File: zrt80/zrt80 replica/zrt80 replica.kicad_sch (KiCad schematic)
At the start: 108 parts, among them J1 VIDEO, J2 POWER, J3 KEYBOARD, J4 S2-S3, J5 RS232, J6 CHAR, J7 RAM, Q1 2N2222, Q2 2N5484, Y1 20MHz, Y2 2.4576MHz

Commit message: schematic 'done'
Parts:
- removed J5: RS232, symbol Connector_Generic:Conn_02x13_Odd_Even
- added J5: RS232, Connector_PinHeader_2.54mm:PinHeader_2x13_P2.54mm_Vertical, symbol Connector_Generic:Conn_02x13_Top_Bottom
- C1, C10, C11, C12, C13, C14, C15, C16, C17, C18, C19, C2, C20, C21, C22, C24, C25, C26, C27, C28, C29, C30, C31, C32, C33, C34, C35, C36, C4, C5, C6, C9: footprint (none) -> Evan's parts:C_Disc_D6.0mm_W2.5mm_P6.35mm
- C23: footprint (none) -> Evan's parts:trimmer cap
- C3: footprint (none) -> Capacitor_THT:CP_Radial_D10.0mm_P5.00mm
- C7, C8: footprint (none) -> Capacitor_THT:C_Disc_D4.3mm_W1.9mm_P5.00mm
- D1: footprint (none) -> LED_THT:LED_D5.0mm
- D2: footprint Diode_THT:D_DO-35_SOD27_P7.62mm_Horizontal -> Diode_THT:D_DO-35_SOD27_P12.70mm_Horizontal
- J1: footprint (none) -> Connector_PinHeader_2.54mm:PinHeader_2x05_P2.54mm_Vertical
- J2: footprint (none) -> TerminalBlock_Phoenix:TerminalBlock_Phoenix_MKDS-1,5-8-5.08_1x08_P5.08mm_Horizontal
- J3: footprint (none) -> Connector_PinHeader_2.54mm:PinHeader_2x13_P2.54mm_Vertical
- J4: footprint (none) -> Connector_PinHeader_2.54mm:PinHeader_2x10_P2.54mm_Vertical
- J6: footprint (none) -> Connector_PinHeader_2.54mm:PinHeader_1x03_P2.54mm_Vertical
- J7: footprint (none) -> Connector_PinHeader_2.54mm:PinHeader_1x06_P2.54mm_Vertical
- L1: footprint (none) -> Inductor_THT:L_Axial_L9.5mm_D4.0mm_P15.24mm_Horizontal_Fastron_SMCC
- Q1: footprint Package_TO_SOT_THT:TO-92_Inline -> Package_TO_SOT_THT:TO-5-3
- Q2: footprint TRANS_2N5484 -> Package_TO_SOT_THT:TO-92L_Inline_Wide
- R1, R10, R11, R12, R13, R14, R15, R16, R17, R2, R3, R4, R5, R6, R7, R8, R9: footprint (none) -> Evan's parts:R_Axial_DIN0204_L3.6mm_D1.6mm_P12.7mm_Horizontal
- S1, S2, S3: footprint (none) -> Button_Switch_THT:SW_DIP_SPSTx08_Slide_6.7x21.88mm_W7.62mm_P2.54mm_LowProfile
- TP1: footprint (none) -> TestPoint:TestPoint_Plated_Hole_D2.0mm
- Y1: footprint (none) -> Crystal:Crystal_HC49-U_Vertical
- Y2: footprint (none) -> Crystal:Crystal_HC33-U_Vertical
- Z1, Z16, Z17, Z2, Z28, Z4: footprint (none) -> Package_DIP:DIP-14_W7.62mm
- Z10, Z11, Z18, Z20, Z21, Z22, Z23, Z29, Z37: footprint (none) -> Package_DIP:DIP-16_W7.62mm
- Z12: footprint (none) -> Package_DIP:DIP-40_W15.24mm
- Z14: footprint DIP254P762X469-14 -> Package_DIP:DIP-14_W7.62mm
- Z15: footprint DIP794W45P254L1969H508Q14 -> Package_DIP:DIP-14_W7.62mm
- Z26, Z27: footprint (none) -> Package_DIP:DIP-18_W7.62mm
- Z31, Z36, Z6, Z7, Z9: footprint (none) -> Package_DIP:DIP-20_W7.62mm
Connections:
- net at R16.1: now also C36.2, Z28.9
- net GND: now reaches R16.2
- net GND: now also C1.2, C10.2, C11.2, C12.2, C13.2, C14.2, C15.2, C16.2, C17.2, C18.2, C19.2, C2.2, C21.2, C22.2, C23.2, C24.2, C25.2, C26.2, C27.2, C28.2, C29.2, C3.2, C30.2, C31.2, C32.2, C33.2, C34.2, C35.2, C4.2, C5.2, C6.2, C7.2, C8.2, C9.2, J1.1 (Pin_1), J1.3 (Pin_3), J1.5 (Pin_5), J1.7 (Pin_7), J1.9 (Pin_9), J2.2 (Pin_2), J2.5 (Pin_5), J3.10 (Pin_10), J3.12 (Pin_12), J3.14 (Pin_14), J3.16 (Pin_16), J3.2 (Pin_2), J3.21 (Pin_21), J3.4 (Pin_4), J3.6 (Pin_6), J3.8 (Pin_8), J4.1 (Pin_1), J4.2 (Pin_2), J7.3 (Pin_3), J7.6 (Pin_6), Q2.1, R12.1, R17.2, R6.1, S1.1, S1.2, S1.3, S1.4, S1.5, S1.6, S1.7, S2.1, S2.2, S2.3, S2.4, S2.5, S2.6, S2.7, S2.8, S3.1, S3.2, S3.3, S3.4, S3.5, S3.6, S3.7, S3.8, Z1.7 (GND), Z10.14 (Cext), Z10.6 (Cext), Z10.8 (GND), Z11.8 (GND), Z12.29 (GND), Z13.19 (WR), Z13.20 (GND), Z13.22 (RD), Z13.25 (~{ADS}), Z14.7 (GND), Z15.7 (GND), Z16.7 (GND), Z17.7 (GND), Z18.8 (GND), Z19.1 (GND), Z19.3 (LPSTB), Z2.7 (GND), Z20.15 (E), Z20.8 (GND), Z21.15 (E), Z21.8 (GND), Z22.15 (E), Z22.8 (GND), Z23.15 (E), Z23.8 (GND), Z24.12 (GND), Z25.12 (GND), Z26.9 (Gnd), Z27.9 (Gnd), Z28.7 (GND), Z29.1 (Ds), Z29.6 (CE), Z29.8 (GND), Z30.12 (GND), Z30.18 (~{CE}), Z30.20 (~{OE}/VPP), Z31.1 (OE), Z31.10 (GND), Z32.12 (GND), Z32.20 (~{OE}), Z33.12 (GND), Z33.20 (~{OE}), Z34.12 (GND), Z34.20 (~{OE}), Z35.12 (GND), Z35.20 (~{OE}), Z36.10 (GND), Z37.15 (E), Z37.8 (GND), Z4.7 (GND), Z6.10 (GND), Z7.10 (GND), J5.7 (Pin_7)
- net at C20.1: now also C22.1, R12.2, R13.1, Z13.16 (XIN)
- net at C20.2: now also Y2.1
- net at Y2.2: now also R13.2, Z13.17 (XOUT), Z28.1
- net I/O4: now reaches Z9.1 (OEa)
- net I/O4: now also Z11.11 (O4), Z9.19 (OEb)
- net D3: now reaches Z9.12 (O3a)
- net D3: now also Z12.8 (D3), Z13.4 (D3), Z19.30 (D3), Z24.13 (D3), Z25.13 (D3), Z26.14 (D0), Z36.14 (B4), Z6.12 (O3a), Z7.12 (O3a)
- net D2: now reaches Z9.14 (O2a)
- net D2: now also Z12.12 (D2), Z13.3 (D2), Z19.31 (D2), Z24.11 (D2), Z25.11 (D2), Z26.13 (D1), Z36.11 (B7), Z6.14 (O2a), Z7.14 (O2a)
- net D1: now reaches Z9.16 (O1a)
- net D1: now also Z12.15 (D1), Z13.2 (D1), Z19.32 (D1), Z24.10 (D1), Z25.10 (D1), Z26.12 (D2), Z36.12 (B6), Z6.16 (O1a), Z7.16 (O1a)
- net D0: now reaches Z9.18 (O0a)
- net D0: now also Z12.14 (D0), Z13.1 (D0), Z19.33 (D0), Z24.9 (D0), Z25.9 (D0), Z26.11 (D3), Z36.13 (B5), Z6.18 (O0a), Z7.18 (O0a)
- net +5V: now reaches Z9.20 (VCC)
- net +5V: now also C1.1, C10.1, C11.1, C12.1, C13.1, C14.1, C15.1, C16.1, C17.1, C18.1, C19.1, C2.1, C21.1, C24.1, C25.1, C26.1, C27.1, C28.1, C29.1, C30.1, C31.1, C32.1, C33.1, C34.1, C35.1, C4.1, C5.1, C6.1, C9.1, D2.1 (K), J2.3 (Pin_3), J3.24 (Pin_24), J3.25 (Pin_25), J3.26 (Pin_26), J6.1 (Pin_1), L1.1, Q1.3 (C), R1.2, R10.2, R11.2, R14.2, R15.2, R2.2, R7.2, R8.2, R9.2, Z1.14 (VCC), Z10.10 (B), Z10.11 (Clr), Z10.16 (VCC), Z10.2 (B), Z10.3 (Clr), Z11.16 (VCC), Z12.11 (VCC), Z13.12 (CS0), Z13.13 (CS1), Z13.40 (VCC), Z14.14 (VCC), Z16.14 (VCC), Z17.14 (VCC), Z18.16 (VCC), Z19.20 (VCC), Z19.23 (E), Z2.14 (VCC), Z20.16 (VCC), Z21.16 (VCC), Z22.16 (VCC), Z23.16 (VCC), Z24.24 (VCC), Z25.24 (VCC), Z26.18 (Vcc), Z27.18 (Vcc), Z28.14 (VCC), Z29.16 (VCC), Z3.1 (R1.1), Z30.24 (VCC), Z31.20 (VCC), Z32.24 (VCC), Z33.24 (VCC), Z34.24 (VCC), Z35.24 (VCC), Z36.20 (VCC), Z37.16 (VCC), Z4.14 (VCC), Z5.1 (R1.1), Z6.20 (VCC), Z7.20 (VCC), Z8.1 (R1.1)
- net D7: now reaches Z9.3 (O3b)
- net D7: now also Z12.13 (D7), Z13.8 (D7), Z19.26 (D7), Z24.17 (D7), Z25.17 (D7), Z27.14 (D0), Z36.18 (B0), Z6.3 (O3b), Z7.3 (O3b)
- net D6: now reaches Z9.5 (O2b)
- net D6: now also Z12.10 (D6), Z13.7 (D6), Z19.27 (D6), Z24.16 (D6), Z25.16 (D6), Z27.13 (D1), Z36.17 (B1), Z6.5 (O2b), Z7.5 (O2b)
- net D5: now reaches Z9.7 (O1b)
- net D5: now also Z12.9 (D5), Z13.6 (D5), Z19.28 (D5), Z24.15 (D5), Z25.15 (D5), Z27.12 (D2), Z36.16 (B2), Z6.7 (O1b), Z7.7 (O1b)
- net D4: now reaches Z9.9 (O0b)
- net D4: now also Z12.7 (D4), Z13.5 (D4), Z19.29 (D4), Z24.14 (D4), Z25.14 (D4), Z27.11 (D3), Z36.15 (B3), Z6.9 (O0b), Z7.9 (O0b)
- net cSyncPol: now reaches Z3.2 (R1.2)
- net cSyncPol: now also S1.16, Z2.1
- net -12V: now reaches Z15.1 (VCC-)
- net -12V: now also J2.1 (Pin_1), J3.22 (Pin_22), J3.23 (Pin_23)
- net at Z15.10 (3B): now also Z13.32 (~{RTS}), Z15.9 (3A)
- net TxDATA: now reaches Z15.11 (4Y)
- net TxDATA: now also J5.2 (Pin_2)
- net at Z15.12 (4A): now also Z13.11 (SOUT), Z15.13 (4B)
- net +12V: now reaches Z15.14 (VCC_+)
- net +12V: now also J2.4 (Pin_4), J3.19 (Pin_19), J3.20 (Pin_20)
- net at Z15.4 (2A): now also Z13.33 (~{DTR}), Z15.5 (2B)
- net DTR: now reaches Z15.6 (2Y)
- net DTR: now also J5.20 (Pin_20)
- net RTS: now reaches Z15.8 (3Y)
- net RTS: now also J5.4 (Pin_4)
- net bell: now reaches Z10.12 (~{Q})
- net bell: now also Z16.2
- net at Z10.7 (RCext): now also C7.1, R8.1
- net I/O6: now reaches Z10.9 (A)
- net I/O6: now also Z11.9 (O6)
- net RAM A7: now reaches Z33.1 (A7)
- net RAM A7: now also Z22.12 (Zd), Z32.1 (A7), Z34.1 (A7), Z35.1 (A7)
- net RAM D1: now reaches Z33.10 (Q1)
- net RAM D1: now also Z31.4 (D1), Z32.10 (Q1), Z34.10 (Q1), Z35.10 (Q1), Z36.8 (A6)
- net RAM D2: now reaches Z33.11 (Q2)
- net RAM D2: now also Z31.3 (D0), Z32.11 (Q2), Z34.11 (Q2), Z35.11 (Q2), Z36.9 (A7)
- net RAM D3: now reaches Z33.13 (Q3)
- net RAM D3: now also Z31.8 (D3), Z32.13 (Q3), Z34.13 (Q3), Z35.13 (Q3), Z36.6 (A4)
- net RAM D4: now reaches Z33.14 (Q4)
- net RAM D4: now also Z31.13 (D4), Z32.14 (Q4), Z34.14 (Q4), Z35.14 (Q4), Z36.5 (A3)
- net RAM D5: now reaches Z33.15 (Q5)
- net RAM D5: now also Z31.14 (D5), Z32.15 (Q5), Z34.15 (Q5), Z35.15 (Q5), Z36.4 (A2)
- net RAM D6: now reaches Z33.16 (Q6)
- net RAM D6: now also Z31.17 (D6), Z32.16 (Q6), Z34.16 (Q6), Z35.16 (Q6), Z36.3 (A1)
- net RAM D7: now reaches Z33.17 (Q7)
- net RAM D7: now also Z31.18 (D7), Z32.17 (Q7), Z34.17 (Q7), Z35.17 (Q7), Z36.2 (A0)
- net RAM /CS2: now reaches Z33.18 (~{CS})
- net RAM /CS2: now also Z37.10 (O2)
- net RAM A10: now reaches Z33.19 (A10)
- net RAM A10: now also Z21.9 (Zc), Z32.19 (A10), Z34.19 (A10), Z35.19 (A10)
- net RAM A6: now reaches Z33.2 (A6)
- net RAM A6: now also Z22.9 (Zc), Z32.2 (A6), Z34.2 (A6), Z35.2 (A6)
- net RAM /WR: now reaches Z33.21 (~{WE})
- net RAM /WR: now also Z21.12 (Zd), Z32.21 (~{WE}), Z34.21 (~{WE}), Z35.21 (~{WE})
- net RAM A9: now reaches Z33.22 (A9)
- net RAM A9: now also Z21.7 (Zb), Z32.22 (A9), Z34.22 (A9), Z35.22 (A9)
- net RAM A8: now reaches Z33.23 (A8)
- net RAM A8: now also Z21.4 (Za), Z32.23 (A8), Z34.23 (A8), Z35.23 (A8)
- net RAM A5: now reaches Z33.3 (A5)
- net RAM A5: now also Z22.7 (Zb), Z32.3 (A5), Z34.3 (A5), Z35.3 (A5)
- net RAM A4: now reaches Z33.4 (A4)
- net RAM A4: now also Z22.4 (Za), Z32.4 (A4), Z34.4 (A4), Z35.4 (A4)
- net RAM A3: now reaches Z33.5 (A3)
- net RAM A3: now also Z23.12 (Zd), Z32.5 (A3), Z34.5 (A3), Z35.5 (A3)
- net RAM A2: now reaches Z33.6 (A2)
- net RAM A2: now also Z23.9 (Zc), Z32.6 (A2), Z34.6 (A2), Z35.6 (A2)
- net RAM A1: now reaches Z33.7 (A1)
- net RAM A1: now also Z23.7 (Zb), Z32.7 (A1), Z34.7 (A1), Z35.7 (A1)
- net RAM A0: now reaches Z33.8 (A0)
- net RAM A0: now also Z23.4 (Za), Z32.8 (A0), Z34.8 (A0), Z35.8 (A0)
- net RAM D0: now reaches Z33.9 (Q0)
- net RAM D0: now also Z31.7 (D2), Z32.9 (Q0), Z34.9 (Q0), Z35.9 (Q0), Z36.7 (A5)
- net SW2-2: now reaches Z5.2 (R1.2)
- net SW2-2: now also J4.14 (Pin_14), S2.15, Z5.3 (R2.2)
- net at R1.1: now also D1.2 (A)
- net at Z13.10 (SIN): now also Z14.6 (OUT_B)
- net I/O0: now reaches Z13.14 (~{CS2})
- net I/O0: now also Z11.15 (O0)
- net at Z13.15 (~{BAUDOUT}): now also Z13.9 (RCLK)
- net /WR: now reaches Z13.18 (~{WR})
- net /WR: now also Z12.22 (~{WR}), Z19.22 (R/~{W}), Z21.14 (I0d), Z26.10 (R/~{W}), Z27.10 (R/~{W}), Z36.1 (A->B)
- net /RD: now reaches Z13.21 (~{RD})
- net /RD: now also Z12.21 (~{RD})
- net A2: now reaches Z13.26 (A2)
- net A2: now also Z12.32 (A2), Z23.11 (I0c), Z24.6 (A2), Z25.6 (A2), Z26.7 (A2), Z27.7 (A2)
- net A1: now reaches Z13.27 (A1)
- net A1: now also Z12.31 (A1), Z23.5 (I0b), Z24.7 (A1), Z25.7 (A1), Z26.6 (A1), Z27.6 (A1)
- net A0: now reaches Z13.28 (A0)
- net A0: now also Z12.30 (A0), Z19.24 (RS), Z23.2 (I0a), Z24.8 (A0), Z25.8 (A0), Z26.5 (A0), Z27.5 (A0)
- net at Z13.30 (INTR): now also Z28.5
- net CA11: now reaches Z13.31 (~{OUT2})
- net CA11: now also J6.3 (Pin_3)
- net at Z13.34 (~{OUT1}): now also Z16.12, Z16.13
- net RESET: now reaches Z13.35 (MR)
- net RESET: now also Z4.11, Z4.12
- net at Z13.36 (~{CTS}): now also Z14.8 (OUT_C)
- net at Z13.37 (~{DSR}): now also Z14.3 (OUT_A)
- net at Z13.38 (~{DCD}): now also Z14.11 (OUT_D)
- net caps lock: now reaches Z13.39 (~{RI})
- net caps lock: now also J3.18 (Pin_18), J4.3 (Pin_3), Z8.10 (R9.2)
- net at Z16.4: now also Z1.12 (Q3), Z1.8 (Cp0)
- net CRTC CLK: now reaches Z16.5
- net CRTC CLK: now also Z1.5 (Q0), Z19.21 (CLK)
- net at Z16.6: now also Z18.9 (Cp), Z4.9
- net SW2-8: now reaches Z5.10 (R9.2)
- net SW2-8: now also J4.8 (Pin_8), S2.9
- net at J6.2 (Pin_2): now also Z30.21 (A11)
- net at Z2.2: now also Z17.3, Z4.5
- net Csync Out: now reaches Z2.3
- net Csync Out: now also J1.8 (Pin_8)
- net at Z3.6 (R5.2): now also Z1.1 (Pl), Z1.13 (Mr)
- net at R4.1: now also Z4.6
- net at R4.2: now also Q1.2 (B), R3.2
- net SW2-4: now reaches J4.10 (Pin_10)
- net SW2-4: now also S2.13, Z5.6 (R5.2)
- net SW3-5: now reaches J4.11 (Pin_11)
- net SW3-5: now also S3.12, Z8.9 (R8.2)
- net SW2-3: now reaches J4.12 (Pin_12)
- net SW2-3: now also S2.14, Z5.5 (R4.2)
- net SW3-1: now reaches J4.13 (Pin_13)
- net SW3-1: now also S3.16, Z8.2 (R1.2)
- net SW3-2: now reaches J4.15 (Pin_15)
- net SW3-2: now also S3.15, Z8.4 (R3.2)
- net SW2-1: now reaches J4.16 (Pin_16)
- net SW2-1: now also S2.16
- net SW3-3: now reaches J4.17 (Pin_17)
- net SW3-3: now also S3.14, Z8.6 (R5.2)
- net SW2-5: now reaches J4.18 (Pin_18)
- net SW2-5: now also S2.12, Z5.7 (R6.2)
- net SW3-4: now reaches J4.19 (Pin_19)
- net SW3-4: now also S3.13, Z8.8 (R7.2)
- net SW2-6: now reaches J4.20 (Pin_20)
- net SW2-6: now also S2.11, Z5.8 (R7.2)
- net EXRESET: now reaches J4.4 (Pin_4)
- net EXRESET: now also C3.1, D2.2 (A), J2.6 (Pin_6), R14.1, S1.11, Z4.13
- net SW3-8: now reaches J4.5 (Pin_5)
- net SW3-8: now also S3.9, Z8.3 (R2.2)
- net SW2-7: now reaches J4.6 (Pin_6)
- net SW2-7: now also S2.10, Z5.9 (R8.2)
- net SW3-7: now reaches J4.7 (Pin_7)
- net SW3-7: now also S3.10, Z8.5 (R4.2)
- net SW3-6: now reaches J4.9 (Pin_9)
- net SW3-6: now also S3.11, Z8.7 (R6.2)
- net hSyncPol: now reaches Z3.7 (R6.2)
- net hSyncPol: now also S1.12, Z2.10
- net KBD0: now reaches J3.1 (Pin_1)
- net KBD0: now also Z7.2 (I0a)
- net KBD5: now reaches J3.11 (Pin_11)
- net KBD5: now also Z7.13 (I1b)
- net KBD6: now reaches J3.13 (Pin_13)
- net KBD6: now also Z7.15 (I2b)
- net ALT: now reaches J3.15 (Pin_15)
- net ALT: now also S1.13, Z3.5 (R4.2), Z7.17 (I3b)
- net KBD STB: now reaches J3.17 (Pin_17)
- net KBD STB: now also Z17.13
- net KBD1: now reaches J3.3 (Pin_3)
- net KBD1: now also Z7.4 (I1a)
- net KBD2: now reaches J3.5 (Pin_5)
- net KBD2: now also Z7.6 (I2a)
- net KBD3: now reaches J3.7 (Pin_7)
- net KBD3: now also Z7.8 (I3a)
- net KBD4: now reaches J3.9 (Pin_9)
- net KBD4: now also Z7.11 (I0b)
- net at Z1.6 (Cp1): now also R2.1, Z28.8
- net Earth_Protective: now reaches TP1.1
- net Earth_Protective: now also J5.1 (Pin_1)
- net A6: now reaches Z27.1 (A6)
- net A6: now also Z12.36 (A6), Z22.11 (I0c), Z24.2 (A6), Z25.2 (A6), Z26.1 (A6)
- net A9: now reaches Z27.15 (A9)
- net A9: now also Z12.39 (A9), Z21.5 (I0b), Z24.22 (A9), Z25.22 (A9), Z26.15 (A9)
- net A8: now reaches Z27.16 (A8)
- net A8: now also Z12.38 (A8), Z21.2 (I0a), Z24.23 (A8), Z25.23 (A8), Z26.16 (A8)
- net A7: now reaches Z27.17 (A7)
- net A7: now also Z12.37 (A7), Z22.14 (I0d), Z24.1 (A7), Z25.1 (A7), Z26.17 (A7)
- net A5: now reaches Z27.2 (A5)
- net A5: now also Z11.3 (A2), Z12.35 (A5), Z22.5 (I0b), Z24.3 (A5), Z25.3 (A5), Z26.2 (A5)
- net A4: now reaches Z27.3 (A4)
- net A4: now also Z11.2 (A1), Z12.34 (A4), Z22.2 (I0a), Z24.4 (A4), Z25.4 (A4), Z26.3 (A4)
- net A3: now reaches Z27.4 (A3)
- net A3: now also Z11.1 (A0), Z12.33 (A3), Z23.14 (I0d), Z24.5 (A3), Z25.5 (A3), Z26.4 (A3)
- net /mem1: now reaches Z27.8 (~{CS})
- net /mem1: now also Z26.8 (~{CS}), Z37.5 (O1)
- net KSTB Pol: now reaches S1.10
- net KSTB Pol: now also Z17.12, Z3.8 (R7.2)
- net vidPol: now reaches S1.14
- net vidPol: now also Z2.12, Z3.4 (R3.2)
- net vSyncPol: now reaches S1.15
- net vSyncPol: now also Z2.4, Z3.3 (R2.2)
- net beep in: now reaches S1.8
- net beep in: now also Z16.3
- net beep out: now reaches S1.9
- net beep out: now also J2.8 (Pin_8)
- net at C23.1: now also C36.1, L1.2, Q2.2, Y1.2
- net /mem0: now reaches Z25.18 (~{CE})
- net /mem0: now also Z24.18 (~{CE}), Z37.4 (O0)
- net A10: now reaches Z25.19 (A10)
- net A10: now also Z12.40 (A10), Z21.11 (I0c), Z24.19 (A10)
- net A12: now reaches Z25.20 (~{OE}/VPP)
- net A12: now also Z12.2 (A12), Z20.5 (I0b), Z28.11
- net A11: now reaches Z25.21 (A11)
- net A11: now also Z12.1 (A11), Z20.2 (I0a), Z24.21 (A11)
- net at Y1.1: now also Q2.3, R17.1
- net I/O3: now reaches Z6.1 (OEa)
- net I/O3: now also Z11.12 (O3), Z6.19 (OEb)
- net phi: now reaches Z28.2
- net phi: now also R15.1, Z12.6 (~{CLK}), Z28.3
- net at R3.1: now also Z4.4
- net CURSOR: now reaches Z17.10
- net CURSOR: now also Z19.19 (CURSOR)
- net at Z17.8: now also Z18.4 (D0)
- net at Z17.9: now also Z31.19 (O7)
- net /phi: now reaches Z28.4
- net DSR: now reaches Z14.1 (IN_A)
- net DSR: now also J5.6 (Pin_6)
- net CTS: now reaches Z14.10 (IN_C)
- net CTS: now also J5.5 (Pin_5)
- net at Z14.12 (RESPONSE_COTROL_D): now also R9.1
- net RLSD: now reaches Z14.13 (IN_D)
- net RLSD: now also J5.8 (Pin_8)
- net at Z14.2 (RESPONSE_COTROL_A): now also R10.1
- net RxDATA: now reaches Z14.4 (IN_B)
- net RxDATA: now also J5.3 (Pin_3)
- net at Z28.10: now also Z24.20 (~{OE}/VPP)
- net at Z4.1: now also Z16.8, Z2.13
- net at Z4.2: now also Z4.3
- net /INT: now reaches Z28.6
- net /INT: now also Z12.16 (~{INT})
- net Vsync: now reaches Z17.1
- net Vsync: now also Z19.40 (VS), Z2.5
- net Hsync: now reaches Z17.2
- net Hsync: now also Z19.39 (HS), Z2.9
- net at Z17.11: now also Z12.17 (~{NMI})
- net Video Out: now reaches Z2.11
- net Video Out: now also J1.2 (Pin_2)
- net /mem3: now reaches Z22.1 (S)
- net /mem3: now also Z18.5 (D1), Z20.1 (S), Z21.1 (S), Z23.1 (S), Z36.19 (CE), Z37.7 (O3)
- net CRTC A6: now reaches Z22.10 (I1c)
- net CRTC A6: now also Z19.10 (MA6)
- net CRTC A7: now reaches Z22.13 (I1d)
- net CRTC A7: now also Z19.11 (MA7)
- net CRTC A4: now reaches Z22.3 (I1a)
- net CRTC A4: now also Z19.8 (MA4)
- net CRTC A5: now reaches Z22.6 (I1b)
- net CRTC A5: now also Z19.9 (MA5)
- net at Z30.1 (A7): now also Z31.9 (O3)
- net at Z30.10 (D1): now also Z29.3 (B)
- net at Z30.11 (D2): now also Z29.4 (C)
- net at Z30.13 (D3): now also Z29.5 (D)
- net at Z30.14 (D4): now also Z29.10 (E)
- net at Z30.15 (D5): now also Z29.11 (F)
- net at Z30.16 (D6): now also Z29.12 (G)
- net at Z30.17 (D7): now also Z29.14 (H)
- net at Z30.19 (A10): now also Z31.16 (O6)
- net at Z30.2 (A6): now also Z31.2 (O0)
- net at Z30.22 (A9): now also Z31.15 (O5)
- net at Z30.23 (A8): now also Z31.12 (O4)
- net at Z30.3 (A5): now also Z31.5 (O1)
- net at Z30.4 (A4): now also Z31.6 (O2)
- net RA3: now reaches Z30.5 (A3)
- net RA3: now also Z19.35 (RA3)
- net RA2: now reaches Z30.6 (A2)
- net RA2: now also Z19.36 (RA2)
- net RA1: now reaches Z30.7 (A1)
- net RA1: now also Z19.37 (RA1)
- net RA0: now reaches Z30.8 (A0)
- net RA0: now also Z19.38 (RA0)
- net at Z30.9 (D0): now also Z29.2 (A)
- net at R11.1: now also Z12.25 (~{BUSRQ})
- net RAM /CS0: now reaches Z35.18 (~{CS})
- net RAM /CS0: now also Z37.12 (O0)
- net at Z17.4: now also Z18.2 (Q0)
- net raw video: now reaches Z17.5
- net raw video: now also Z29.13 (Qh)
- net at Z17.6: now also Z16.9
- net Vsync Out: now reaches Z2.6
- net Vsync Out: now also J1.6 (Pin_6)
- net I/O7: now reaches Z10.1 (A)
- net I/O7: now also Z11.7 (O7)
- net at Z10.15 (RCext): now also C8.1, R7.1
- net beep: now reaches Z10.4 (~{Q})
- net beep: now also Z16.1
- net /RESET: now reaches Z4.10
- net /RESET: now also Z12.26 (~{RESET})
- net at R5.1: now also Q1.1 (E), R6.2
- net composite video: now reaches R5.2
- net composite video: now also J1.10 (Pin_10)
- net at Z5.4 (R3.2): now also Z21.13 (I1d)
- net CRTC A13: now reaches Z20.10 (I1c)
- net CRTC A13: now also Z19.17 (MA13)
- net A13: now reaches Z20.11 (I0c)
- net A13: now also Z12.3 (A13)
- net CRTC A11: now reaches Z20.3 (I1a)
- net CRTC A11: now also Z19.15 (MA11)
- net RAM A11: now reaches Z20.4 (Za)
- net RAM A11: now also J7.1 (Pin_1)
- net CRTC A12: now reaches Z20.6 (I1b)
- net CRTC A12: now also Z19.16 (MA12)
- net RAM A12: now reaches Z20.7 (Zb)
- net RAM A12: now also J7.4 (Pin_4)
- net CRTC A8: now reaches Z19.12 (MA8)
- net CRTC A8: now also Z21.3 (I1a)
- net CRTC A9: now reaches Z19.13 (MA9)
- net CRTC A9: now also Z21.6 (I1b)
- net CRTC A10: now reaches Z19.14 (MA10)
- net CRTC A10: now also Z21.10 (I1c)
- net DE: now reaches Z19.18 (DE)
- net DE: now also Z18.13 (D3)
- net /reset: now reaches Z19.2 (~{RESET})
- net I/O1: now reaches Z19.25 (~{CS})
- net I/O1: now also Z11.14 (O1)
- net CRTC A0: now reaches Z19.4 (MA0)
- net CRTC A0: now also Z23.3 (I1a)
- net CRTC A1: now reaches Z19.5 (MA1)
- net CRTC A1: now also Z23.6 (I1b)
- net CRTC A2: now reaches Z19.6 (MA2)
- net CRTC A2: now also Z23.10 (I1c)
- net CRTC A3: now reaches Z19.7 (MA3)
- net CRTC A3: now also Z23.13 (I1d)
- net I/O5: now reaches Z11.10 (O5)
- net I/O2: now reaches Z11.13 (O2)
- net I/O2: now also Z7.1 (OEa), Z7.19 (OEb)
- net ~{M1}: now reaches Z11.4 (E1)
- net ~{M1}: now also Z12.27 (~{M1})
- net ~{IO REQ}: now reaches Z11.5 (E2)
- net ~{IO REQ}: now also Z11.6 (E3), Z12.20 (~{IORQ})
- net RAM /CS3: now reaches Z32.18 (~{CS})
- net RAM /CS3: now also Z37.9 (O3)
- net Hsync Out: now reaches Z2.8
- net Hsync Out: now also J1.4 (Pin_4)
- net LED: now reaches Z16.11
- net LED: now also D1.1 (K), J2.7 (Pin_7)
- net at Z4.8: now also Z29.15 (PE), Z31.11 (Cp)
- net /MREQ: now reaches Z12.19 (~{MREQ})
- net /MREQ: now also Z37.1 (E)
- net at Z12.24 (~{WAIT}): now also Z3.9 (R8.2)
- net A14: now reaches Z12.4 (A14)
- net A14: now also Z37.2 (A0)
- net A15: now reaches Z12.5 (A15)
- net A15: now also Z37.3 (A1)
- net /mem2: now reaches Z37.6 (O2)
- net at J7.2 (Pin_2): now also Z37.14 (A0)
- net at J7.5 (Pin_5): now also Z37.13 (A1)
- net RAM /CS1: now reaches Z34.18 (~{CS})
- net RAM /CS1: now also Z37.11 (O1)
- net DOT CLK: now reaches Z29.7 (Clk)
- net DEGLCH: now reaches Z29.9 (Clr)
- net DEGLCH: now also Z18.10 (Q2)
- net blanking: now reaches Z16.10
- net blanking: now also Z18.15 (Q3)
- net at Z18.1 (~{Mr}): now also Z3.10 (R9.2)
- net at Z18.12 (D2): now also Z18.7 (Q1)
- no-connect marks 0 -> 43
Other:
- moved on the sheet: C1, C10, C11, C12, C13, C14, C15, C16, C17, C18, C19, C2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

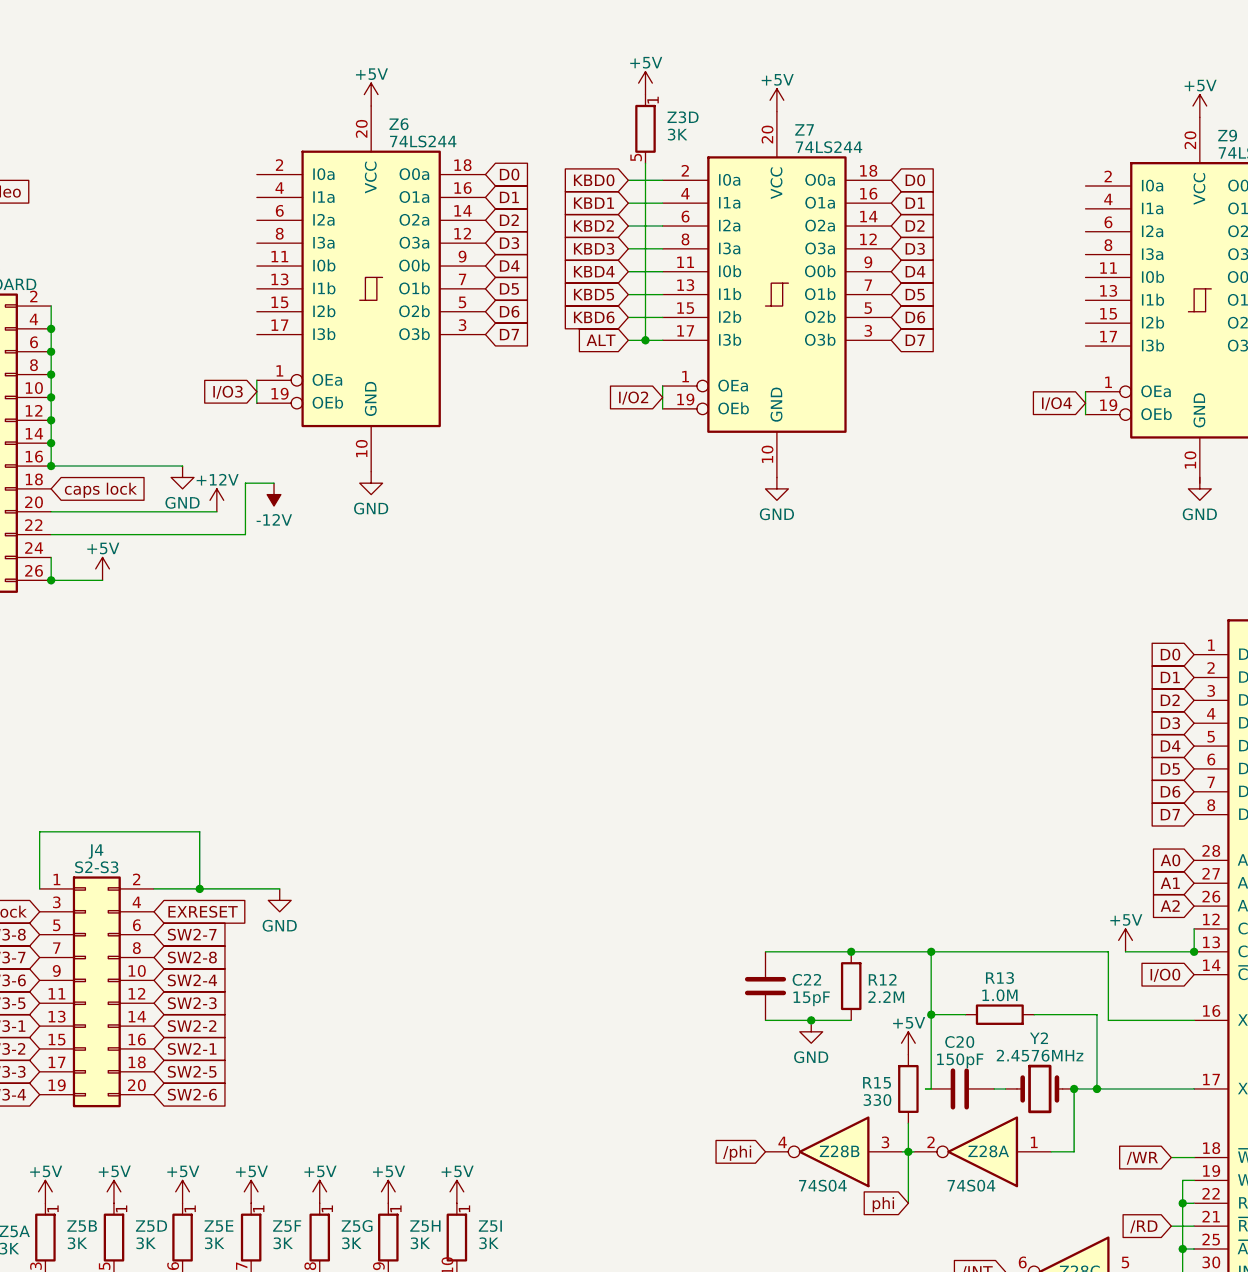
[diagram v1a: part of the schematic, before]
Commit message: layout for zrt80 progressing
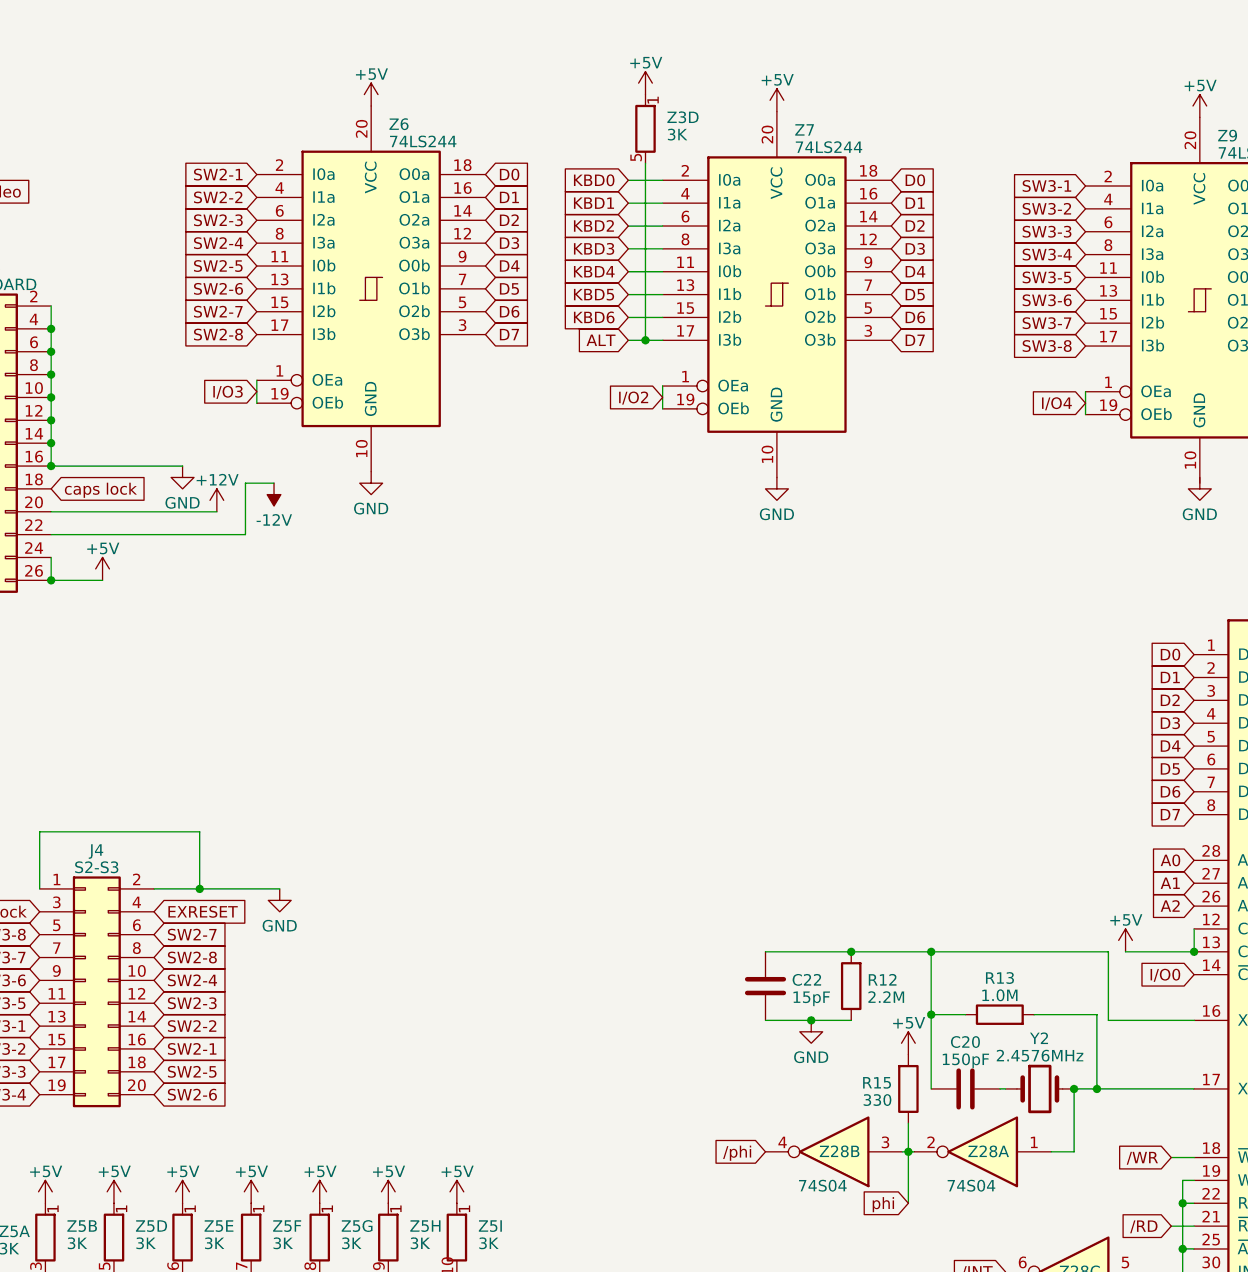
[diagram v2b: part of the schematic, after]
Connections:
- net SW2-1: now also Z6.2 (I0a)
- net SW2-2: now also Z6.4 (I1a)
- net SW2-3: now also Z6.6 (I2a)
- net SW2-4: now also Z6.8 (I3a)
- net SW2-5: now also Z6.11 (I0b)
- net SW2-6: now also Z6.13 (I1b)
- net SW2-7: now also Z6.15 (I2b)
- net SW2-8: now also Z6.17 (I3b)
- net SW3-1: now also Z9.2 (I0a)
- net SW3-2: now also Z9.4 (I1a)
- net SW3-3: now also Z9.6 (I2a)
- net SW3-4: now also Z9.8 (I3a)
- net SW3-5: now also Z9.11 (I0b)
- net SW3-6: now also Z9.13 (I1b)
- net SW3-7: now also Z9.15 (I2b)
- net SW3-8: now also Z9.17 (I3b)
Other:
- moved on the sheet: C20
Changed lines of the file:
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@@
     (stroke (width 0) (type default))
   )
-  (wire (pts (xy 389.255 132.08) (xy 388.62 132.08))
-    (stroke (width 0) (type default))
-  )
   (wire (pts (xy 263.525 162.56) (xy 263.525 165.1))
     (stroke (width 0) (type default))
@@
     (stroke (width 0) (type default))
   )
-  (wire (pts (xy 396.24 132.08) (xy 397.51 132.08))
+  (wire (pts (xy 396.875 132.08) (xy 397.51 132.08))
     (stroke (width 0) (type default))
   )
@@
     )
   )
+  (global_label "SW2-1" (shape input) (at 314.325 30.48 180) (fields_autoplaced)
+    (effects (font (size 1.27 1.27)) (justify right))
+    (property "Intersheetrefs" "${INTERSHEET_REFS}" (at 304.7669 30.48 0)
+      (effects (font (size 1.27 1.27)) (justify right) hide)
+    )
+  )
   (global_label "Hsync Out" (shape input) (at 272.415 24.765 0) (fields_autoplaced)
     (effects (font (size 1.27 1.27)) (justify left))
@@
     )
   )
+  (global_label "SW3-4" (shape input) (at 406.4 39.37 180) (fields_autoplaced)
+    (effects (font (size 1.27 1.27)) (justify right))
+    (property "Intersheetrefs" "${INTERSHEET_REFS}" (at 396.8419 39.37 0)
+      (effects (font (size 1.27 1.27)) (justify right) hide)
+    )
+  )
   (global_label "RAM D4" (shape input) (at 189.865 302.26 0) (fields_autoplaced)
     (effects (font (size 1.27 1.27)) (justify left))
@@
     )
   )
+  (global_label "SW3-7" (shape input) (at 406.4 46.99 180) (fields_autoplaced)
+    (effects (font (size 1.27 1.27)) (justify right))
+    (property "Intersheetrefs" "${INTERSHEET_REFS}" (at 396.8419 46.99 0)
+      (effects (font (size 1.27 1.27)) (justify right) hide)
+    )
+  )
   (global_label "RAM A0" (shape input) (at 164.465 292.1 180) (fields_autoplaced)
     (effects (font (size 1.27 1.27)) (justify right))
@@
     )
   )
+  (global_label "SW3-8" (shape input) (at 406.4 49.53 180) (fields_autoplaced)
+    (effects (font (size 1.27 1.27)) (justify right))
+    (property "Intersheetrefs" "${INTERSHEET_REFS}" (at 396.8419 49.53 0)
+      (effects (font (size 1.27 1.27)) (justify right) hide)
+    )
+  )
   (global_label "RAM D7" (shape input) (at 189.865 309.88 0) (fields_autoplaced)
     (effects (font (size 1.27 1.27)) (justify left))
@@
     )
   )
+  (global_label "SW2-8" (shape input) (at 314.325 48.26 180) (fields_autoplaced)
+    (effects (font (size 1.27 1.27)) (justify right))
+    (property "Intersheetrefs" "${INTERSHEET_REFS}" (at 304.7669 48.26 0)
+      (effects (font (size 1.27 1.27)) (justify right) hide)
+    )
+  )
   (global_label "RAM A10" (shape input) (at 229.87 193.675 0) (fields_autoplaced)
     (effects (font (size 1.27 1.27)) (justify left))
@@
     )
   )
+  (global_label "SW3-3" (shape input) (at 406.4 36.83 180) (fields_autoplaced)
+    (effects (font (size 1.27 1.27)) (justify right))
+    (property "Intersheetrefs" "${INTERSHEET_REFS}" (at 396.8419 36.83 0)
+      (effects (font (size 1.27 1.27)) (justify right) hide)
+    )
+  )
   (global_label "DEGLCH" (shape input) (at 79.375 100.965 0) (fields_autoplaced)
     (effects (font (size 1.27 1.27)) (justify left))
@@
     )
   )
+  (global_label "SW2-3" (shape input) (at 314.325 35.56 180) (fields_autoplaced)
+    (effects (font (size 1.27 1.27)) (justify right))
+    (property "Intersheetrefs" "${INTERSHEET_REFS}" (at 304.7669 35.56 0)
+      (effects (font (size 1.27 1.27)) (justify right) hide)
+    )
+  )
   (global_label "{slash}mem3" (shape input) (at 223.52 97.155 180) (fields_autoplaced)
     (effects (font (size 1.27 1.27)) (justify right))
@@
     )
   )
+  (global_label "SW3-6" (shape input) (at 406.4 44.45 180) (fields_autoplaced)
+    (effects (font (size 1.27 1.27)) (justify right))
+    (property "Intersheetrefs" "${INTERSHEET_REFS}" (at 396.8419 44.45 0)
+      (effects (font (size 1.27 1.27)) (justify right) hide)
+    )
+  )
   (global_label "A1" (shape input) (at 483.235 297.815 180) (fields_autoplaced)
     (effects (font (size 1.27 1.27)) (justify right))
@@
     )
   )
+  (global_label "SW2-5" (shape input) (at 314.325 40.64 180) (fields_autoplaced)
+    (effects (font (size 1.27 1.27)) (justify right))
+    (property "Intersheetrefs" "${INTERSHEET_REFS}" (at 304.7669 40.64 0)
+      (effects (font (size 1.27 1.27)) (justify right) hide)
+    )
+  )
   (global_label "D7" (shape input) (at 355.6 298.45 0) (fields_autoplaced)
     (effects (font (size 1.27 1.27)) (justify left))
@@
     )
   )
+  (global_label "SW3-2" (shape input) (at 406.4 34.29 180) (fields_autoplaced)
+    (effects (font (size 1.27 1.27)) (justify right))
+    (property "Intersheetrefs" "${INTERSHEET_REFS}" (at 396.8419 34.29 0)
+      (effects (font (size 1.27 1.27)) (justify right) hide)
+    )
+  )
   (global_label "RAM D7" (shape input) (at 155.575 215.9 0) (fields_autoplaced)
     (effects (font (size 1.27 1.27)) (justify left))
@@
     )
   )
+  (global_label "SW3-5" (shape input) (at 406.4 41.91 180) (fields_autoplaced)
+    (effects (font (size 1.27 1.27)) (justify right))
+    (property "Intersheetrefs" "${INTERSHEET_REFS}" (at 396.8419 41.91 0)
+      (effects (font (size 1.27 1.27)) (justify right) hide)
+    )
+  )
   (global_label "CRTC A12" (shape input) (at 179.705 142.875 0) (fields_autoplaced)
     (effects (font (size 1.27 1.27)) (justify left))
@@
     )
   )
+  (global_label "SW2-7" (shape input) (at 314.325 45.72 180) (fields_autoplaced)
+    (effects (font (size 1.27 1.27)) (justify right))
+    (property "Intersheetrefs" "${INTERSHEET_REFS}" (at 304.7669 45.72 0)
+      (effects (font (size 1.27 1.27)) (justify right) hide)
+    )
+  )
   (global_label "D0" (shape input) (at 339.725 30.48 0) (fields_autoplaced)
     (effects (font (size 1.27 1.27)) (justify left))
@@
     )
   )
+  (global_label "SW2-6" (shape input) (at 314.325 43.18 180) (fields_autoplaced)
+    (effects (font (size 1.27 1.27)) (justify right))
+    (property "Intersheetrefs" "${INTERSHEET_REFS}" (at 304.7669 43.18 0)
+      (effects (font (size 1.27 1.27)) (justify right) hide)
+    )
+  )
   (global_label "D3" (shape input) (at 431.8 39.37 0) (fields_autoplaced)
     (effects (font (size 1.27 1.27)) (justify left))
@@
     )
   )
+  (global_label "SW2-4" (shape input) (at 314.325 38.1 180) (fields_autoplaced)
+    (effects (font (size 1.27 1.27)) (justify right))
+    (property "Intersheetrefs" "${INTERSHEET_REFS}" (at 304.7669 38.1 0)
+      (effects (font (size 1.27 1.27)) (justify right) hide)
+    )
+  )
   (global_label "{slash}WR" (shape input) (at 379.73 328.295 270) (fields_autoplaced)
     (effects (font (size 1.27 1.27)) (justify right))
@@
     )
   )
+  (global_label "SW3-1" (shape input) (at 406.4 31.75 180) (fields_autoplaced)
+    (effects (font (size 1.27 1.27)) (justify right))
+    (property "Intersheetrefs" "${INTERSHEET_REFS}" (at 396.8419 31.75 0)
+      (effects (font (size 1.27 1.27)) (justify right) hide)
+    )
+  )
   (global_label "RLSD" (shape input) (at 509.27 78.74 0) (fields_autoplaced)
     (effects (font (size 1.27 1.27)) (justify left))
@@
     )
   )
+  (global_label "SW2-2" (shape input) (at 314.325 33.02 180) (fields_autoplaced)
+    (effects (font (size 1.27 1.27)) (justify right))
+    (property "Intersheetrefs" "${INTERSHEET_REFS}" (at 304.7669 33.02 0)
+      (effects (font (size 1.27 1.27)) (justify right) hide)
+    )
+  )
   (global_label "I{slash}O4" (shape input) (at 406.4 55.88 180) (fields_autoplaced)
     (effects (font (size 1.27 1.27)) (justify right))
@@
     )
   )
-  (symbol (lib_id "Device:C") (at 392.43 132.08 90) (unit 1)
+  (symbol (lib_id "Device:C") (at 393.065 132.08 90) (unit 1)
     (in_bom yes) (on_board yes) (dnp no) (fields_autoplaced)
-    (property "Reference" "C20" (at 392.43 126.9111 90)
+    (property "Reference" "C20" (at 393.065 126.9111 90)
       (effects (font (size 1.27 1.27)))
     )
-    (property "Value" "150pF" (at 392.43 128.8321 90)
+    (property "Value" "150pF" (at 393.065 128.8321 90)
       (effects (font (size 1.27 1.27)))
     )
-    (property "Footprint" "Evan's parts:C_Disc_D6.0mm_W2.5mm_P6.35mm" (at 396.24 131.1148 0)
+    (property "Footprint" "Evan's parts:C_Disc_D6.0mm_W2.5mm_P6.35mm" (at 396.875 131.1148 0)
       (effects (font (size 1.27 1.27)) hide)
     )
-    (property "Datasheet" "~" (at 392.43 132.08 0)
+    (property "Datasheet" "~" (at 393.065 132.08 0)
       (effects (font (size 1.27 1.27)) hide)
     )
